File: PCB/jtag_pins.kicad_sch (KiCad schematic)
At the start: 3 parts, among them Y1 40MHz

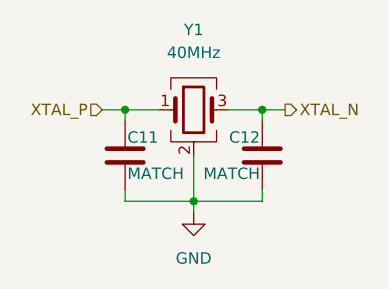
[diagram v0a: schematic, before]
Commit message: yeah just read the journal son
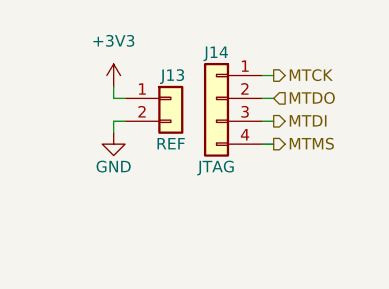
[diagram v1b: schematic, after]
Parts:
- removed C11, C12: MATCH, Capacitor_SMD:C_0603_1608Metric, symbol Device:C
- removed Y1: 40MHz, symbol Device:Crystal_GND24
- added J13: REF, Connector_PinHeader_2.54mm:PinHeader_1x02_P2.54mm_Vertical, symbol Connector_Generic:Conn_01x02
- added J14: JTAG, Connector_PinHeader_2.54mm:PinHeader_1x04_P2.54mm_Vertical, symbol Connector_Generic:Conn_01x04
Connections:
- net GND: now also J13.2 (Pin_2)
- new net +3V3: J13.1 (Pin_1)
- new net MTCK: J14.1 (Pin_1)
- new net MTDI: J14.3 (Pin_3)
- new net MTDO: J14.2 (Pin_2)
- new net MTMS: J14.4 (Pin_4)
